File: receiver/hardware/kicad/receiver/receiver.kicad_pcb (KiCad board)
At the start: 2 copper layers, 20.1 x 63.8 mm, 27 parts, among them J1 Connector, U1 74HC595, U2 74HC595

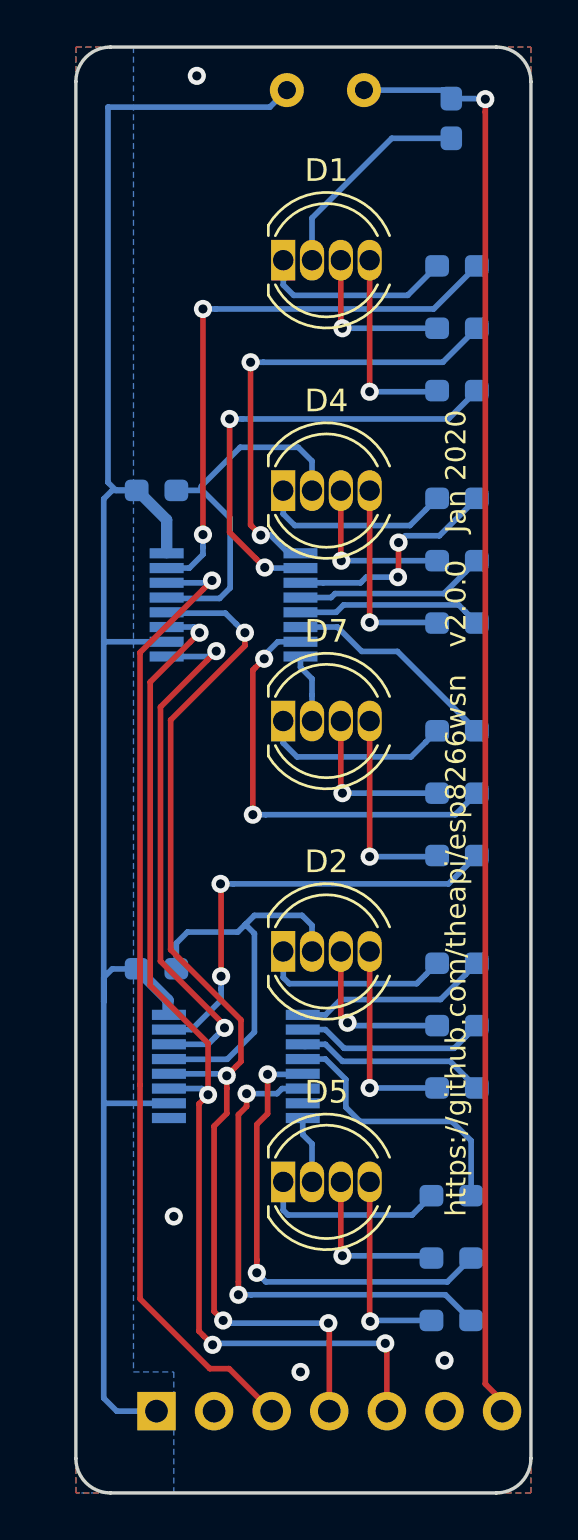
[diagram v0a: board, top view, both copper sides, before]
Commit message: Logos
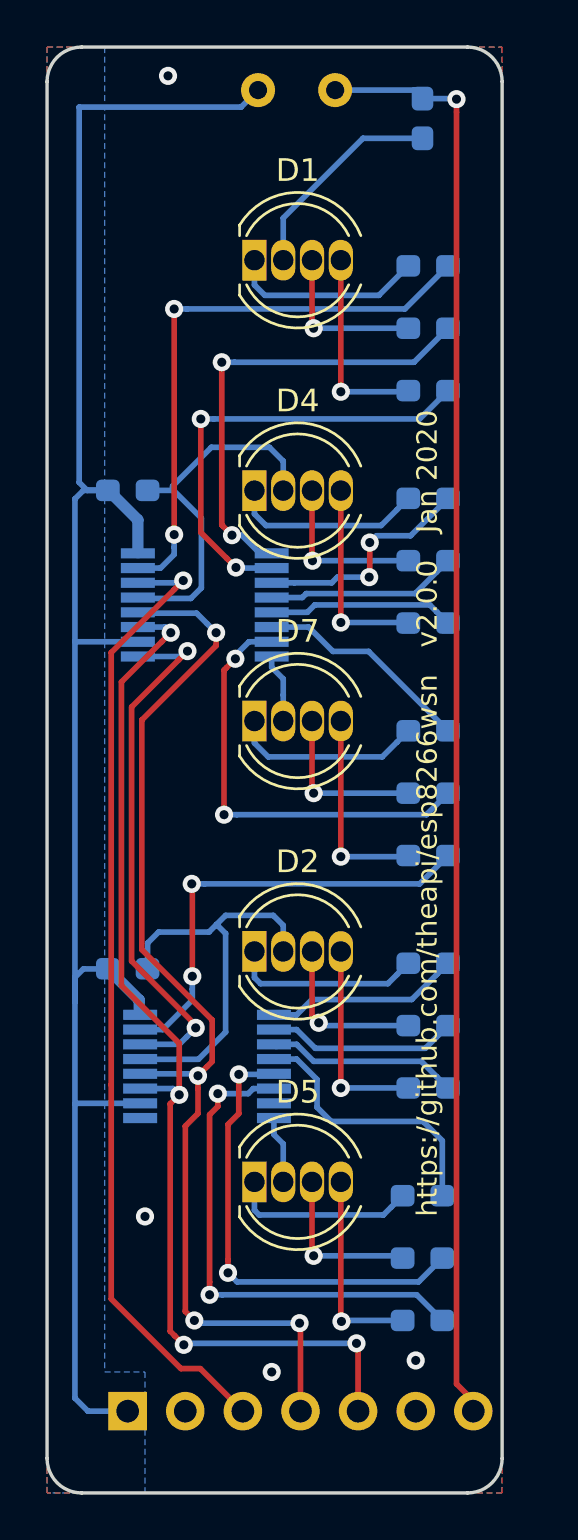
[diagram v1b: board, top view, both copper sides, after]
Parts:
- added REF**: TheApiLogoTiny, theapi:TheApiLogoTiny, F.Cu at (142.7, 56.8)
- added REF**: TheApiLogoTiny, theapi:TheApiLogoTiny, B.Cu at (142.7, 56.8)
- moved C1 1.27 mm to (141.7, 73.7)
- moved C2 1.27 mm to (141.7, 94.7)
- moved D1 1.27 mm to (147.3, 63.5)
- moved D2 1.27 mm to (147.3, 94.0)
- moved D4 1.27 mm to (147.3, 73.7)
- moved D5 1.27 mm to (147.3, 104.1)
- moved D7 1.27 mm to (147.3, 83.8)
- moved J1 1.27 mm to (141.7, 114.2)
- moved R1 1.27 mm to (147.5, 56.0)
- moved R10 1.27 mm to (155.0, 100.0)
- moved R12 1.27 mm to (155.0, 74.0)
- moved R13 1.27 mm to (154.7, 104.8)
- moved R15 1.27 mm to (155.0, 76.8)
- moved R16 1.27 mm to (154.7, 107.5)
- moved R18 1.27 mm to (155.0, 79.5)
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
